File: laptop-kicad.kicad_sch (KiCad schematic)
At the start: 25 parts, among them P1 USB_C_Plug, SW1 SW_Push, U1 ATmega32U4-M, Y1 16MHz

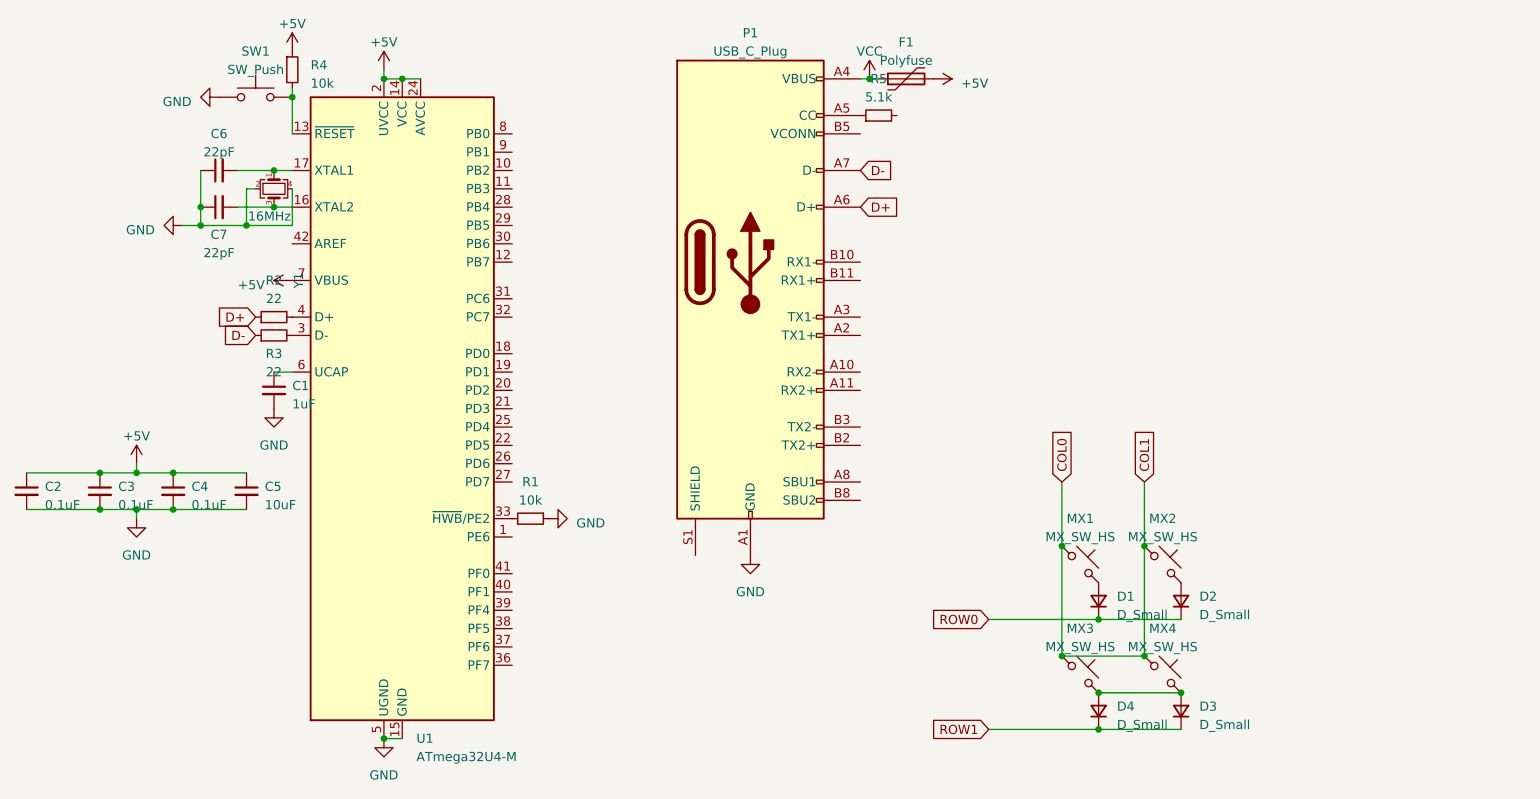
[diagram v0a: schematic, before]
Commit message: D
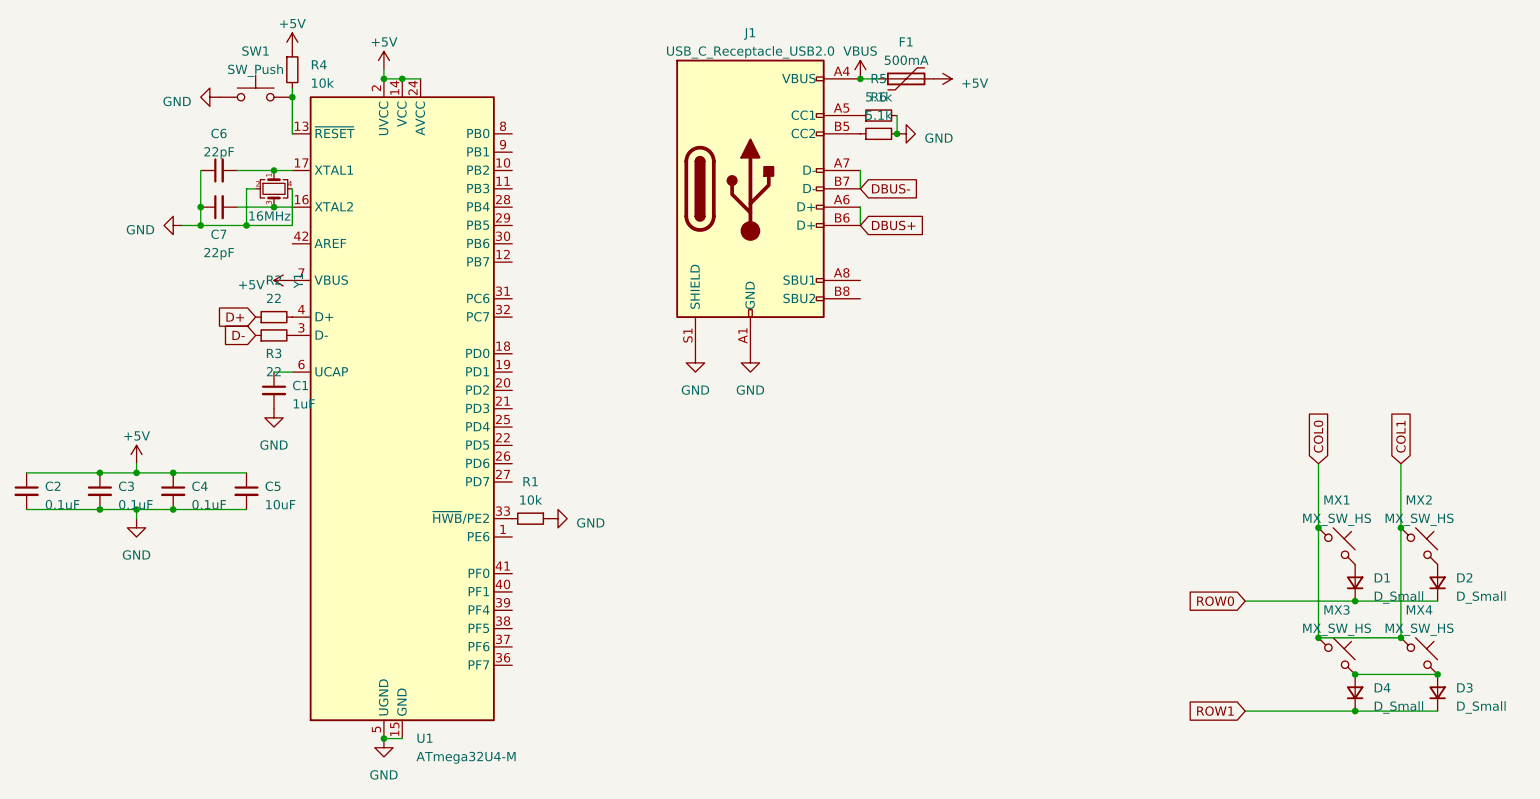
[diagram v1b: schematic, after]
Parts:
- removed P1: USB_C_Plug, Connector_USB:USB_C_Plug_JAE_DX07P024AJ1, symbol Connector:USB_C_Plug
- added J1: USB_C_Receptacle_USB2.0, Connector_USB:USB_C_Receptacle_G-Switch_GT-USB-7010ASV, symbol Connector:USB_C_Receptacle_USB2.0
- added R6: 5.1k, Resistor_SMD:R_0805_2012Metric, symbol Device:R_Small
- F1: value Polyfuse -> 500mA
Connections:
- net GND: now also R5.2, J1.A1 (GND), J1.A12 (GND), J1.B1 (GND), J1.B12 (GND), J1.S1 (SHIELD), R6.2
- net at R5.1: now also J1.A5 (CC1)
- net VCC renamed VBUS
- net VBUS: now also J1.A4 (VBUS), J1.A9 (VBUS), J1.B4 (VBUS), J1.B9 (VBUS)
- new net: J1.B5 (CC2), R6.1
- new net DBUS+: J1.A6 (D+), J1.B6 (D+)
- new net DBUS-: J1.A7 (D-), J1.B7 (D-)
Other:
- moved on the sheet: D1, D2, D3, D4, MX1, MX2, MX3, MX4

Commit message: redoing everything
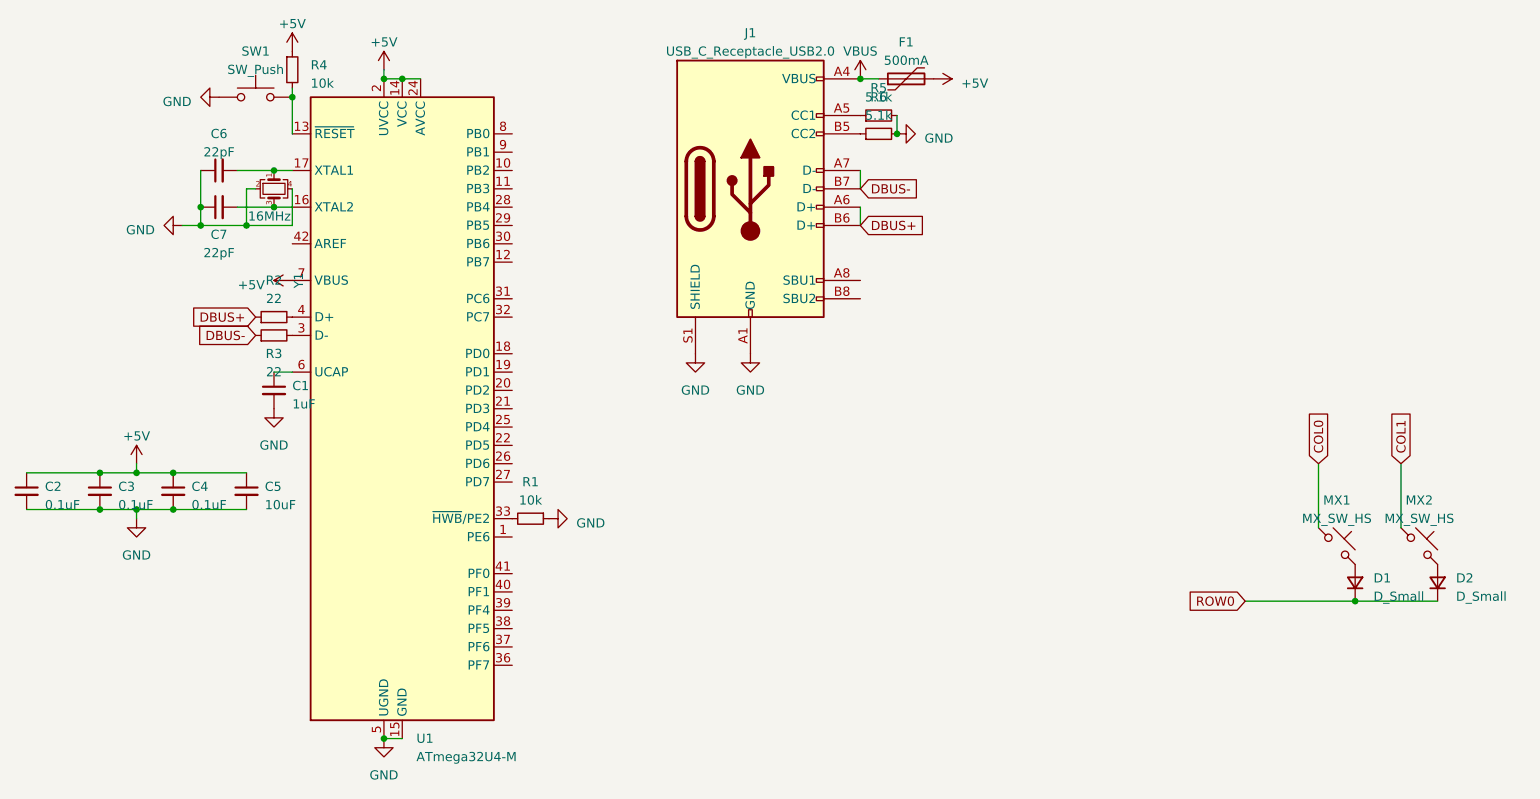
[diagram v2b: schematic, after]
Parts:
- removed D3, D4: D_Small, Diode_SMD:D_SOD-123, symbol Device:D_Small
- removed MX3, MX4: MX_SW_HS, PCM_marbastlib-mx:SW_MX_HS_1u, symbol PCM_marbastlib-mx:MX_SW_HS
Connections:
- net D+ is gone; now on net DBUS+: R2.1
- net D- is gone; now on net DBUS-: R3.1
- net COL0: no longer MX2.1
- new net COL1: MX2.1
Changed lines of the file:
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@@
 (kicad_sch (version 20230121) (generator eeschema)
   (paper "A4")
-  (junction (at 229.87 115.57) (diameter 0) (color 0 0 0 0)
-  )
   (junction (at 100.33 129.54) (diameter 0) (color 0 0 0 0)
   )
@@
   (junction (at 85.09 50.8) (diameter 0) (color 0 0 0 0)
   )
-  (junction (at 229.87 100.33) (diameter 0) (color 0 0 0 0)
-  )
   (junction (at 171.45 45.72) (diameter 0) (color 0 0 0 0)
   )
-  (junction (at 246.38 120.65) (diameter 0) (color 0 0 0 0)
-  )
   (junction (at 102.87 38.1) (diameter 0) (color 0 0 0 0)
   )
@@
   (junction (at 85.09 55.88) (diameter 0) (color 0 0 0 0)
   )
-  (junction (at 234.95 125.73) (diameter 0) (color 0 0 0 0)
-  )
-  (junction (at 234.95 120.65) (diameter 0) (color 0 0 0 0)
-  )
   (junction (at 66.04 97.79) (diameter 0) (color 0 0 0 0)
   )
@@
   (junction (at 71.12 92.71) (diameter 0) (color 0 0 0 0)
   )
-  (junction (at 241.3 100.33) (diameter 0) (color 0 0 0 0)
-  )
   (junction (at 71.12 97.79) (diameter 0) (color 0 0 0 0)
   )
-  (junction (at 241.3 115.57) (diameter 0) (color 0 0 0 0)
-  )
   (junction (at 87.63 40.64) (diameter 0) (color 0 0 0 0)
   )
@@
     (stroke (width 0) (type default))
   )
-  (wire (pts (xy 241.3 115.57) (xy 241.3 100.33))
-    (stroke (width 0) (type default))
-  )
   (wire (pts (xy 229.87 91.44) (xy 229.87 100.33))
     (stroke (width 0) (type default))
@@
     (stroke (width 0) (type default))
   )
-  (wire (pts (xy 234.95 125.73) (xy 219.71 125.73))
-    (stroke (width 0) (type default))
-  )
   (wire (pts (xy 87.63 58.42) (xy 81.28 58.42))
     (stroke (width 0) (type default))
   )
-  (wire (pts (xy 234.95 125.73) (xy 246.38 125.73))
-    (stroke (width 0) (type default))
-  )
   (wire (pts (xy 234.95 110.49) (xy 246.38 110.49))
     (stroke (width 0) (type default))
@@
     (stroke (width 0) (type default))
   )
-  (wire (pts (xy 246.38 120.65) (xy 234.95 120.65))
-    (stroke (width 0) (type default))
-  )
-  (wire (pts (xy 229.87 100.33) (xy 229.87 115.57))
-    (stroke (width 0) (type default))
-  )
   (wire (pts (xy 85.09 50.8) (xy 87.63 50.8))
     (stroke (width 0) (type default))
@@
   )
   (wire (pts (xy 81.28 58.42) (xy 81.28 53.34))
-    (stroke (width 0) (type default))
-  )
-  (wire (pts (xy 229.87 115.57) (xy 241.3 115.57))
     (stroke (width 0) (type default))
   )
@@
     )
   )
-  (global_label "D-" (shape input) (at 82.55 73.66 180) (fields_autoplaced)
+  (global_label "DBUS-" (shape input) (at 82.55 73.66 180) (fields_autoplaced)
     (effects (font (size 1.27 1.27)) (justify right))
-    (property "Intersheetrefs" "${INTERSHEET_REFS}" (at 76.8018 73.66 0)
+    (property "Intersheetrefs" "${INTERSHEET_REFS}" (at 72.9918 73.66 0)
       (effects (font (size 1.27 1.27)) (justify right) hide)
     )
   )
-  (global_label "D+" (shape input) (at 82.55 71.12 180) (fields_autoplaced)
+  (global_label "DBUS+" (shape input) (at 82.55 71.12 180) (fields_autoplaced)
     (effects (font (size 1.27 1.27)) (justify right))
-    (property "Intersheetrefs" "${INTERSHEET_REFS}" (at 76.8018 71.12 0)
+    (property "Intersheetrefs" "${INTERSHEET_REFS}" (at 72.9918 71.12 0)
       (effects (font (size 1.27 1.27)) (justify right) hide)
     )
@@
     )
   )
-  (global_label "ROW1" (shape input) (at 219.71 125.73 180) (fields_autoplaced)
-    (effects (font (size 1.27 1.27)) (justify right))
-    (property "Intersheetrefs" "${INTERSHEET_REFS}" (at 211.5428 125.73 0)
-      (effects (font (size 1.27 1.27)) (justify right) hide)
-    )
-  )
   (global_label "ROW0" (shape input) (at 219.71 110.49 180) (fields_autoplaced)
     (effects (font (size 1.27 1.27)) (justify right))
@@
   )
   (symbol (lib_id "Device:R_Small") (at 168.91 43.18 90) (unit 1)
-    (in_bom yes) (on_board yes) (dnp no) (fields_autoplaced)
-    (property "Reference" "R5" (at 168.91 38.1 90)
+    (in_bom yes) (on_board yes) (dnp no)
+    (property "Reference" "R5" (at 168.91 39.37 90)
       (effects (font (size 1.27 1.27)))
     )
@@
         (path "/228c3151-edb9-403e-9d91-9515ea5c490d"
           (reference "#PWR010") (unit 1)
-        )
-      )
-    )
-  )
-  (symbol (lib_id "Device:D_Small") (at 234.95 123.19 90) (unit 1)
-    (in_bom yes) (on_board yes) (dnp no) (fields_autoplaced)
-    (property "Reference" "D4" (at 237.49 122.555 90)
-      (effects (font (size 1.27 1.27)) (justify right))
-    )
-    (property "Value" "D_Small" (at 237.49 125.095 90)
-      (effects (font (size 1.27 1.27)) (justify right))
-    )
-    (property "Footprint" "Diode_SMD:D_SOD-123" (at 234.95 123.19 90)
-      (effects (font (size 1.27 1.27)) hide)
-    )
-    (property "Datasheet" "~" (at 234.95 123.19 90)
-      (effects (font (size 1.27 1.27)) hide)
-    )
-    (property "Sim.Device" "D" (at 234.95 123.19 0)
-      (effects (font (size 1.27 1.27)) hide)
-    )
-    (property "Sim.Pins" "1=K 2=A" (at 234.95 123.19 0)
-      (effects (font (size 1.27 1.27)) hide)
-    )
-    (pin "1")
-    (pin "2")
-    (instances
-      (project "laptop-kicad"
-        (path "/228c3151-edb9-403e-9d91-9515ea5c490d"
-          (reference "D4") (unit 1)
         )
       )
@@
         (path "/228c3151-edb9-403e-9d91-9515ea5c490d"
           (reference "Y1") (unit 1)
-        )
-      )
-    )
-  )
-  (symbol (lib_id "Device:D_Small") (at 246.38 123.19 90) (unit 1)
-    (in_bom yes) (on_board yes) (dnp no) (fields_autoplaced)
-    (property "Reference" "D3" (at 248.92 122.555 90)
-      (effects (font (size 1.27 1.27)) (justify right))
-    )
-    (property "Value" "D_Small" (at 248.92 125.095 90)
-      (effects (font (size 1.27 1.27)) (justify right))
-    )
-    (property "Footprint" "Diode_SMD:D_SOD-123" (at 246.38 123.19 90)
-      (effects (font (size 1.27 1.27)) hide)
-    )
-    (property "Datasheet" "~" (at 246.38 123.19 90)
-      (effects (font (size 1.27 1.27)) hide)
-    )
-    (property "Sim.Device" "D" (at 246.38 123.19 0)
-      (effects (font (size 1.27 1.27)) hide)
-    )
-    (property "Sim.Pins" "1=K 2=A" (at 246.38 123.19 0)
-      (effects (font (size 1.27 1.27)) hide)
-    )
-    (pin "1")
-    (pin "2")
-    (instances
-      (project "laptop-kicad"
-        (path "/228c3151-edb9-403e-9d91-9515ea5c490d"
-          (reference "D3") (unit 1)
         )
       )
@@
     )
   )
-  (symbol (lib_id "PCM_marbastlib-mx:MX_SW_HS") (at 243.84 118.11 0) (unit 1)
-    (in_bom yes) (on_board yes) (dnp no) (fields_autoplaced)
-    (property "Reference" "MX4" (at 243.84 111.76 0)
-      (effects (font (size 1.27 1.27)))
-    )
-    (property "Value" "MX_SW_HS" (at 243.84 114.3 0)
-      (effects (font (size 1.27 1.27)))
-    )
-    (property "Footprint" "PCM_marbastlib-mx:SW_MX_HS_1u" (at 243.84 118.11 0)
-      (effects (font (size 1.27 1.27)) hide)
-    )
-    (property "Datasheet" "~" (at 243.84 118.11 0)
-      (effects (font (size 1.27 1.27)) hide)
-    )
-    (pin "1")
-    (pin "2")
-    (instances
-      (project "laptop-kicad"
-        (path "/228c3151-edb9-403e-9d91-9515ea5c490d"
-          (reference "MX4") (unit 1)
-        )
-      )
-    )
-  )
   (symbol (lib_id "power:VBUS") (at 166.37 38.1 0) (unit 1)
     (in_bom yes) (on_board yes) (dnp no) (fields_autoplaced)
@@
         )
       )
-    )
-  )
-  (symbol (lib_id "PCM_marbastlib-mx:MX_SW_HS") (at 232.41 118.11 0) (unit 1)
-    (in_bom yes) (on_board yes) (dnp no) (fields_autoplaced)
-    (property "Reference" "MX3" (at 232.41 111.76 0)
-      (effects (font (size 1.27 1.27)))
-    )
-    (property "Value" "MX_SW_HS" (at 232.41 114.3 0)
-      (effects (font (size 1.27 1.27)))
-    )
-    (property "Footprint" "PCM_marbastlib-mx:SW_MX_HS_1u" (at 232.41 118.11 0)
-      (effects (font (size 1.27 1.27)) hide)
-    )
-    (property "Datasheet" "~" (at 232.41 118.11 0)
-      (effects (font (size 1.27 1.27)) hide)
-    )
-    (pin "1")
-    (pin "2")
-    (instances
-      (project "laptop-kicad"
-        (path "/228c3151-edb9-403e-9d91-9515ea5c490d"
-          (reference "MX3") (unit 1)
-        )
-      )

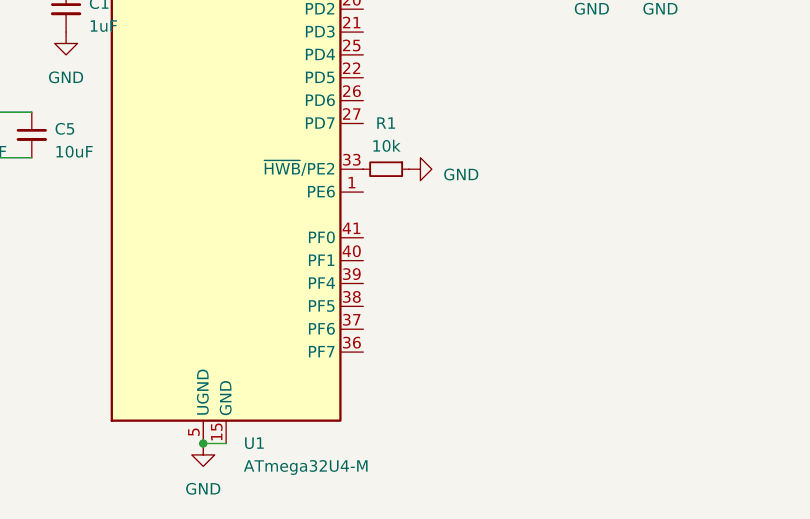
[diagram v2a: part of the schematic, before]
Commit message: PCB is done pt 2
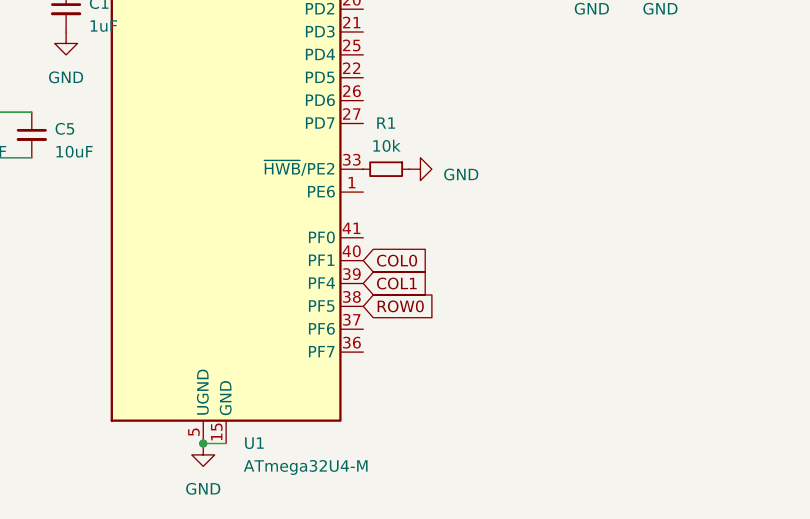
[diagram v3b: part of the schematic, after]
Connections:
- net COL0: now also U1.40 (PF1)
- net COL1: now also U1.39 (PF4)
- net ROW0: now also U1.38 (PF5)
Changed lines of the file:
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@@
+    )
+  )
+  (global_label "ROW0" (shape input) (at 118.11 114.3 0) (fields_autoplaced)
+    (effects (font (size 1.27 1.27)) (justify left))
+    (property "Intersheetrefs" "${INTERSHEET_REFS}" (at 126.2772 114.3 0)
+      (effects (font (size 1.27 1.27)) (justify left) hide)
     )
   )
@@
       (effects (font (size 1.27 1.27)) (justify left) hide)
     )
+  )
+  (global_label "COL0" (shape input) (at 118.11 109.22 0) (fields_autoplaced)
+    (effects (font (size 1.27 1.27)) (justify left))
+    (property "Intersheetrefs" "${INTERSHEET_REFS}" (at 125.8539 109.22 0)
+      (effects (font (size 1.27 1.27)) (justify left) hide)
+    )
+  )
+  (global_label "COL1" (shape input) (at 118.11 111.76 0) (fields_autoplaced)
+    (effects (font (size 1.27 1.27)) (justify left))
+    (property "Intersheetrefs" "${INTERSHEET_REFS}" (at 125.8539 111.76 0)
+      (effects (font (size 1.27 1.27)) (justify left) hide)
+    )
